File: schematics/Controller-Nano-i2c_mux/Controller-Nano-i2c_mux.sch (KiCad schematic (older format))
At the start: 22 parts, among them P1 CONN_02X04, P2 CONN_02X04, P3 CONN_01X04, P4 CONN_01X04, P5 CONN_01X01, P6 CONN_01X01, P7 CONN_01X01, P8 CONN_01X01, U1 Arduino_Nano, U2 PCA9544A

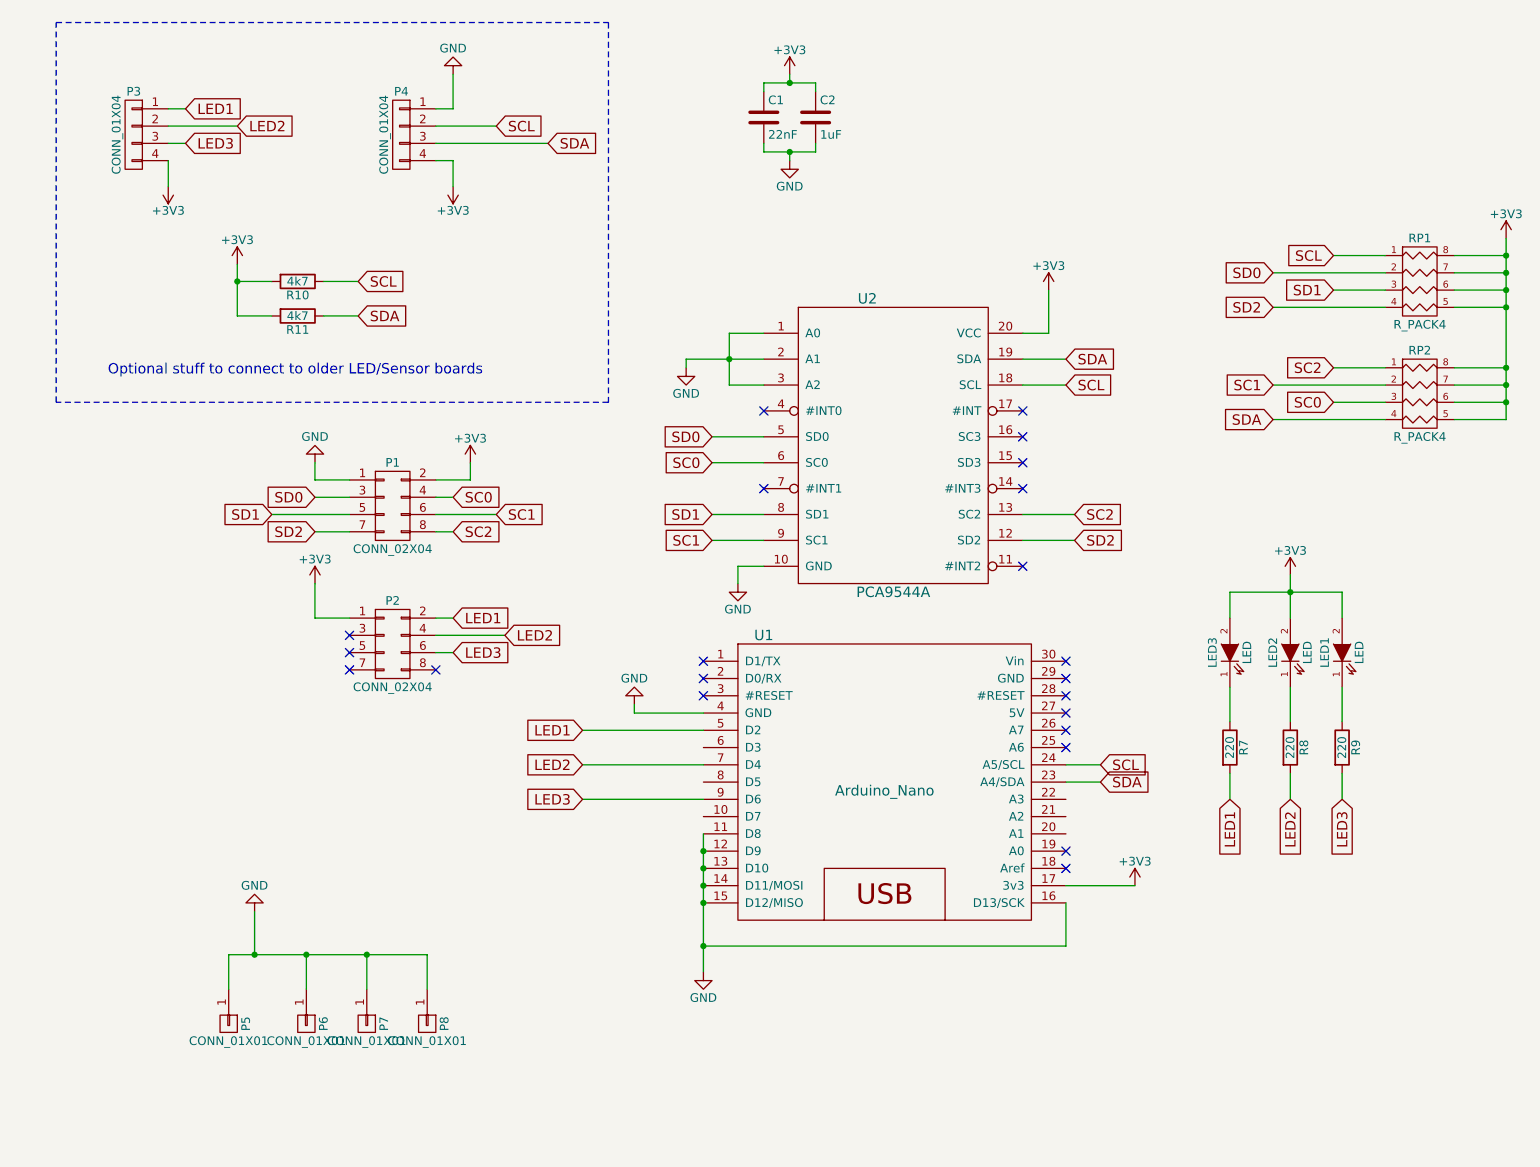
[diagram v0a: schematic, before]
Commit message: Schematics update
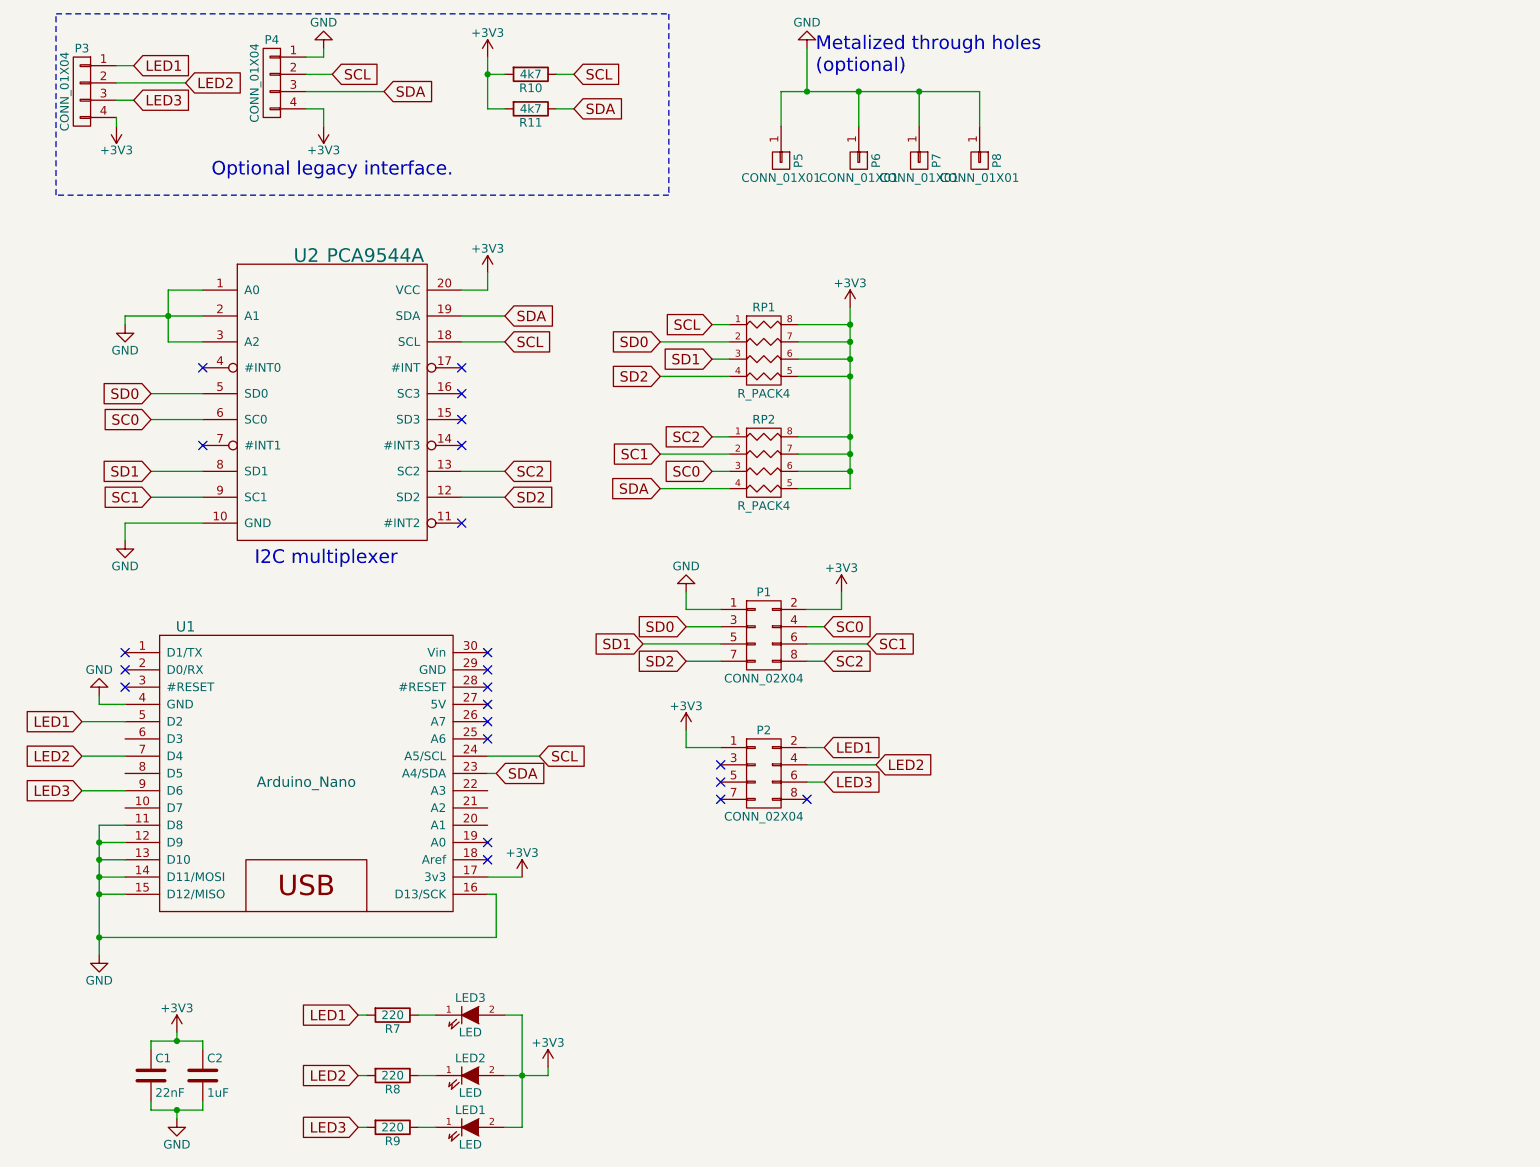
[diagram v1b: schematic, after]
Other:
- note added: "I2C multiplexer"
- note added: "Metalized through holes\n(optional)"
- note added: "Optional legacy interface.\n"
- note removed: "Optional stuff to connect to older LED/Sensor boards\n"
- moved on the sheet: C1, C2, LED1, LED2, LED3, P1, P2, P3, P4, P5, P6, P7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
